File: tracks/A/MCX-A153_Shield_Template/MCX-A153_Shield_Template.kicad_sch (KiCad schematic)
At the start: 8 parts, among them J1 Conn_02x08_Odd_Even, J2 Conn_02x10_Odd_Even, J3 Conn_02x08_Odd_Even

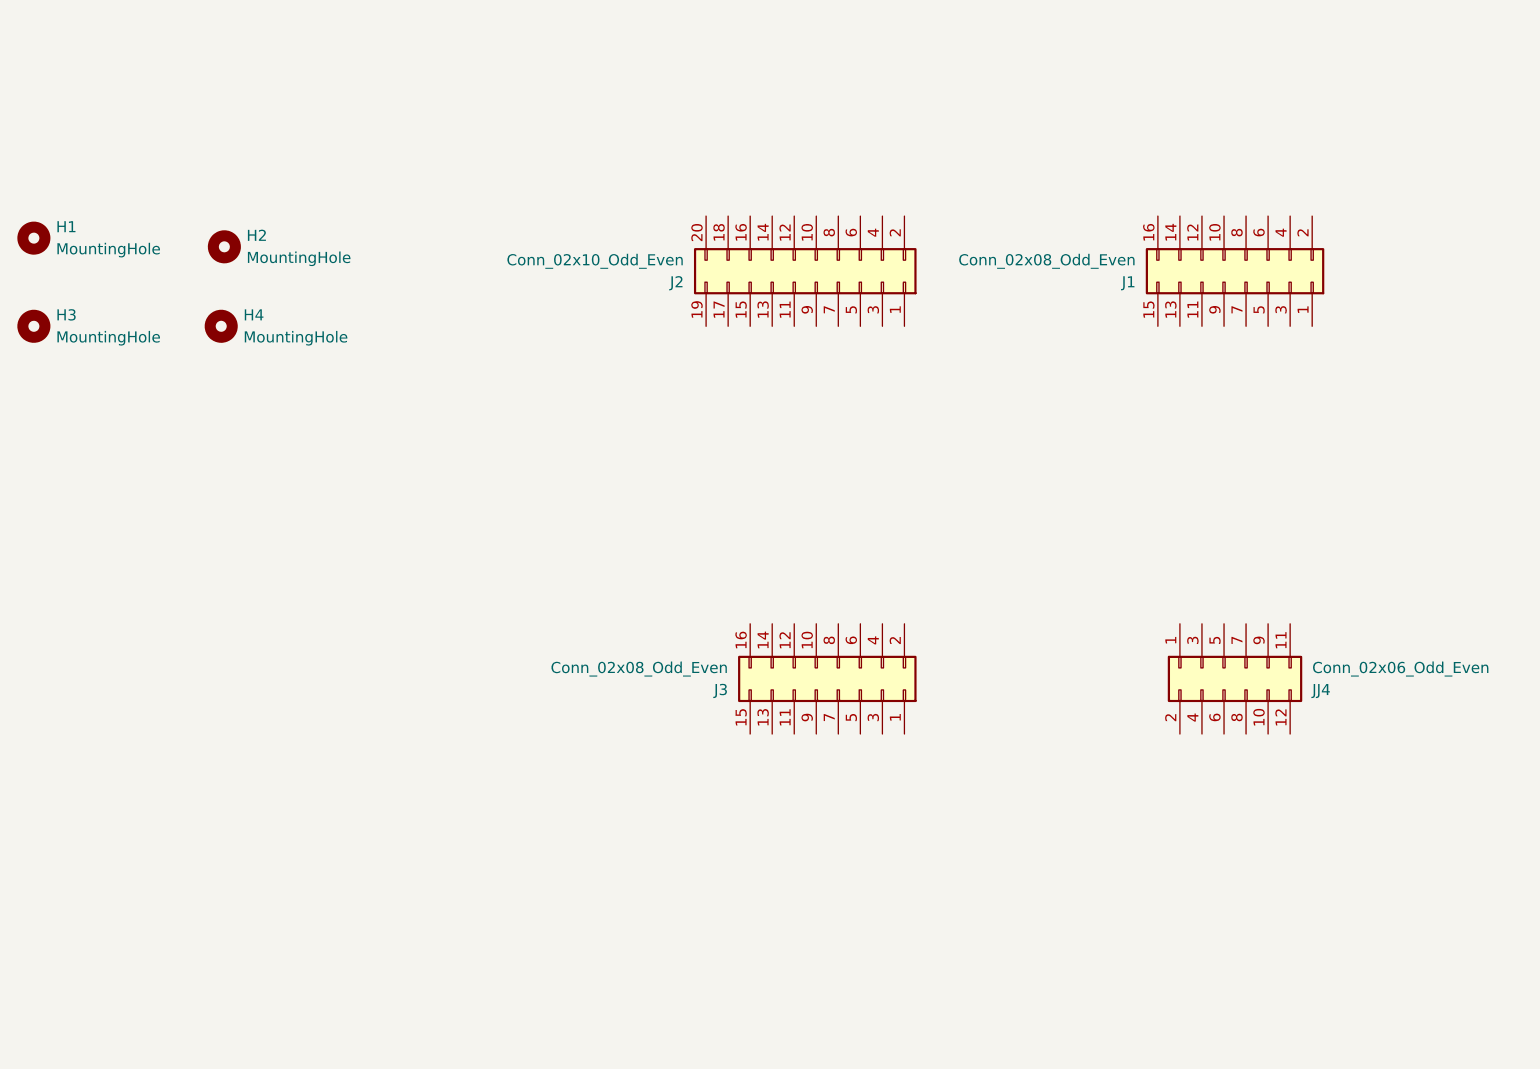
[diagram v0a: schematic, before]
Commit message: -> Added labels to the schematics.
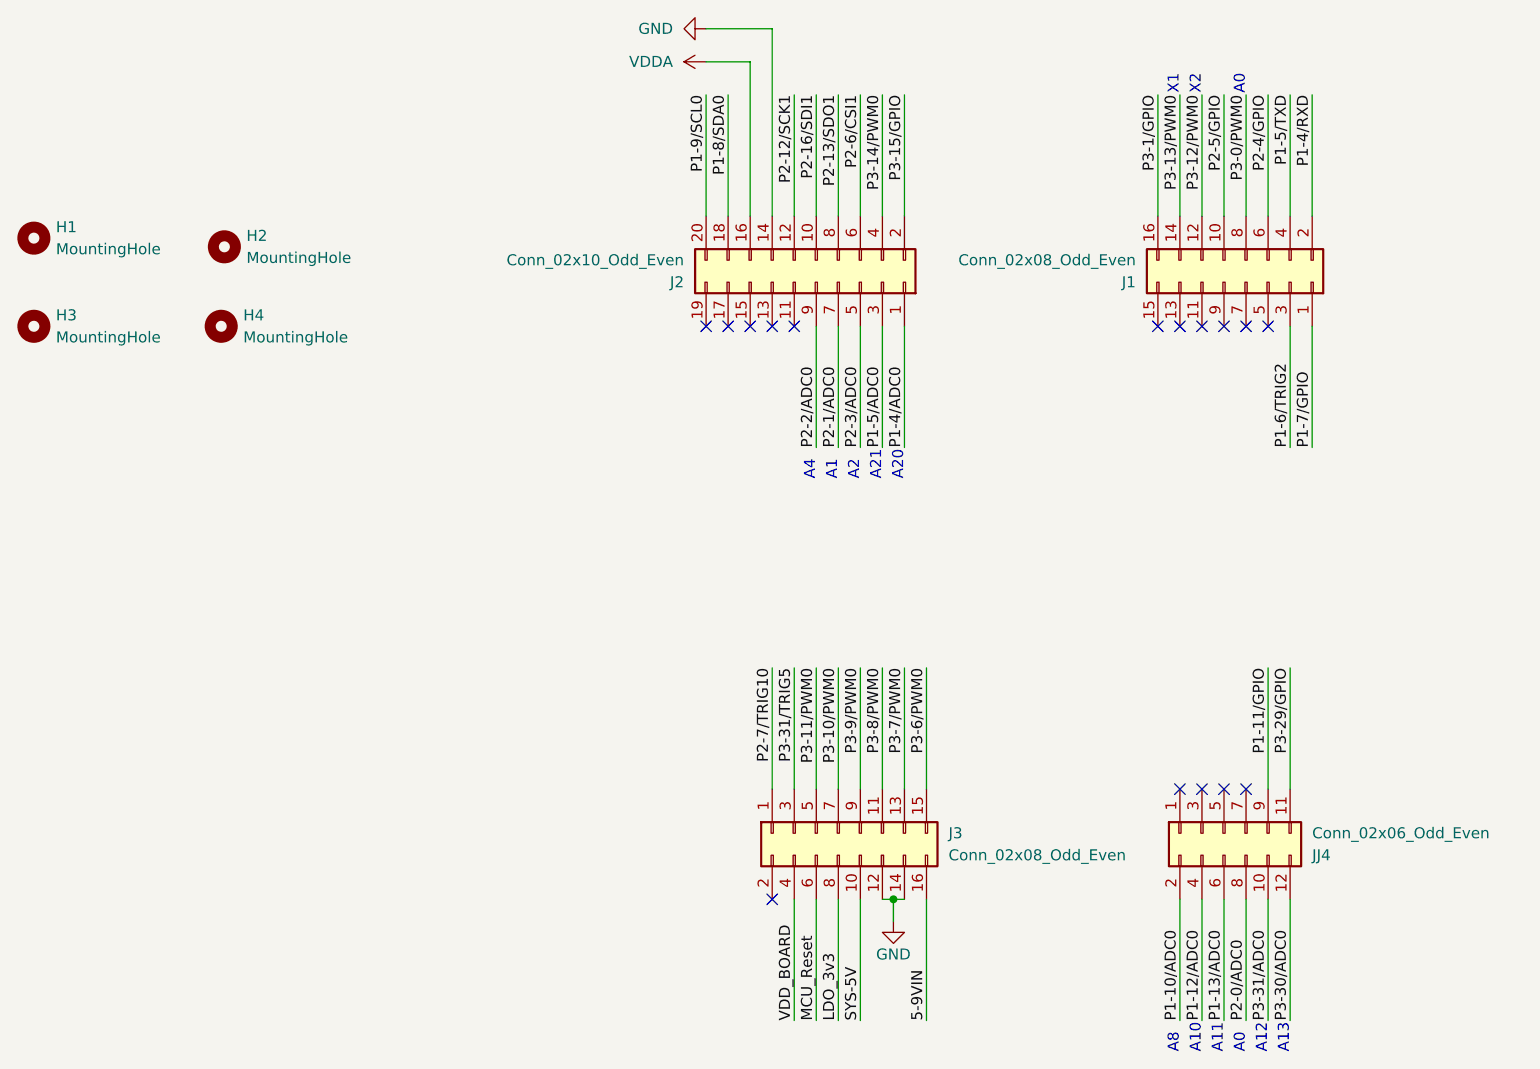
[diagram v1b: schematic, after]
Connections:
- net P1-7/GPIO: now reaches J1.1 (Pin_1)
- net P2-5/GPIO: now reaches J1.10 (Pin_10)
- net P3-12/PWM0: now reaches J1.12 (Pin_12)
- net P3-13/PWM0: now reaches J1.14 (Pin_14)
- net P3-1/GPIO: now reaches J1.16 (Pin_16)
- net P1-4/RXD: now reaches J1.2 (Pin_2)
- net P1-6/TRIG2: now reaches J1.3 (Pin_3)
- net P1-5/TXD: now reaches J1.4 (Pin_4)
- net P2-4/GPIO: now reaches J1.6 (Pin_6)
- net P3-0/PWM0: now reaches J1.8 (Pin_8)
- net P3-31/ADC0: now reaches JJ4.10 (Pin_10)
- net P3-29/GPIO: now reaches JJ4.11 (Pin_11)
- net P3-30/ADC0: now reaches JJ4.12 (Pin_12)
- net P1-10/ADC0: now reaches JJ4.2 (Pin_2)
- net P1-12/ADC0: now reaches JJ4.4 (Pin_4)
- net P1-13/ADC0: now reaches JJ4.6 (Pin_6)
- net P2-0/ADC0: now reaches JJ4.8 (Pin_8)
- net P1-11/GPIO: now reaches JJ4.9 (Pin_9)
- net P2-7/TRIG10: now reaches J3.1 (Pin_1)
- net SYS-5V: now reaches J3.10 (Pin_10)
- net P3-8/PWM0: now reaches J3.11 (Pin_11)
- net GND: now reaches J3.12 (Pin_12)
- net GND: now also J2.14 (Pin_14), J3.14 (Pin_14)
- net P3-7/PWM0: now reaches J3.13 (Pin_13)
- net P3-6/PWM0: now reaches J3.15 (Pin_15)
- net 5-9VIN: now reaches J3.16 (Pin_16)
- net P3-31/TRIG5: now reaches J3.3 (Pin_3)
- net VDD_BOARD: now reaches J3.4 (Pin_4)
- net P3-11/PWM0: now reaches J3.5 (Pin_5)
- net MCU_Reset: now reaches J3.6 (Pin_6)
- net P3-10/PWM0: now reaches J3.7 (Pin_7)
- net LDO_3v3: now reaches J3.8 (Pin_8)
- net P3-9/PWM0: now reaches J3.9 (Pin_9)
- net P1-4/ADC0: now reaches J2.1 (Pin_1)
- net P2-16/SDI1: now reaches J2.10 (Pin_10)
- net P2-12/SCK1: now reaches J2.12 (Pin_12)
- net VDDA: now reaches J2.16 (Pin_16)
- net P1-8/SDA0: now reaches J2.18 (Pin_18)
- net P3-15/GPIO: now reaches J2.2 (Pin_2)
- net P1-9/SCL0: now reaches J2.20 (Pin_20)
- net P1-5/ADC0: now reaches J2.3 (Pin_3)
- net P3-14/PWM0: now reaches J2.4 (Pin_4)
- net P2-3/ADC0: now reaches J2.5 (Pin_5)
- net P2-6/CSI1: now reaches J2.6 (Pin_6)
- net P2-1/ADC0: now reaches J2.7 (Pin_7)
- net P2-13/SDO1: now reaches J2.8 (Pin_8)
- net P2-2/ADC0: now reaches J2.9 (Pin_9)
- no-connect marks 0 -> 16
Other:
- note added: "A0"
- note added: "A1"
- note added: "A10"
- note added: "A11"
- note added: "A12"
- note added: "A13"
- note added: "A2"
- note added: "A20"
- note added: "A21"
- note added: "A4"
- note added: "A8"
- note added: "X1"
- note added: "X2"
- moved on the sheet: J3, JJ4
